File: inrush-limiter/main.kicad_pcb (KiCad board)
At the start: 2 copper layers, 24 parts, among them K1 RELAY_2RT, P1 CONN_01X06, Q1 PN2222A, Q2 PN2222A, U1 LM393

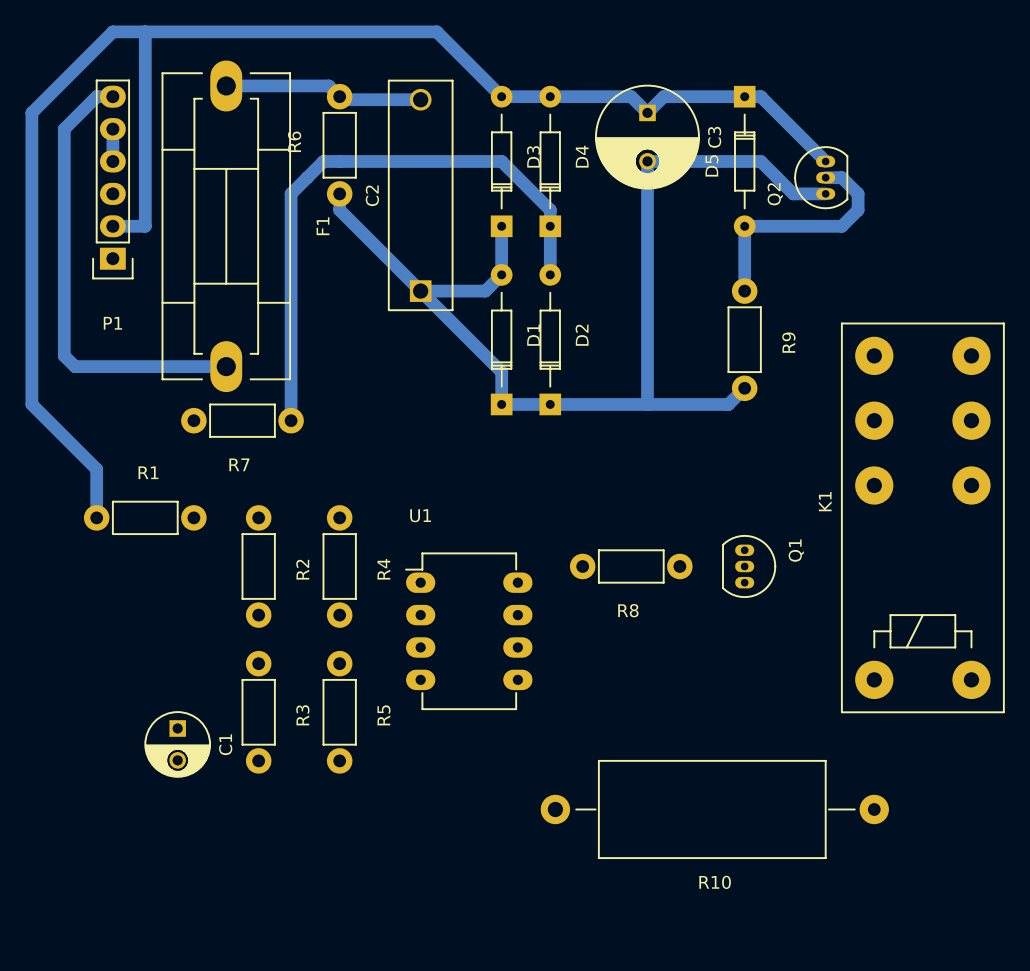
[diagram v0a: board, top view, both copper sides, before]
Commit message: update
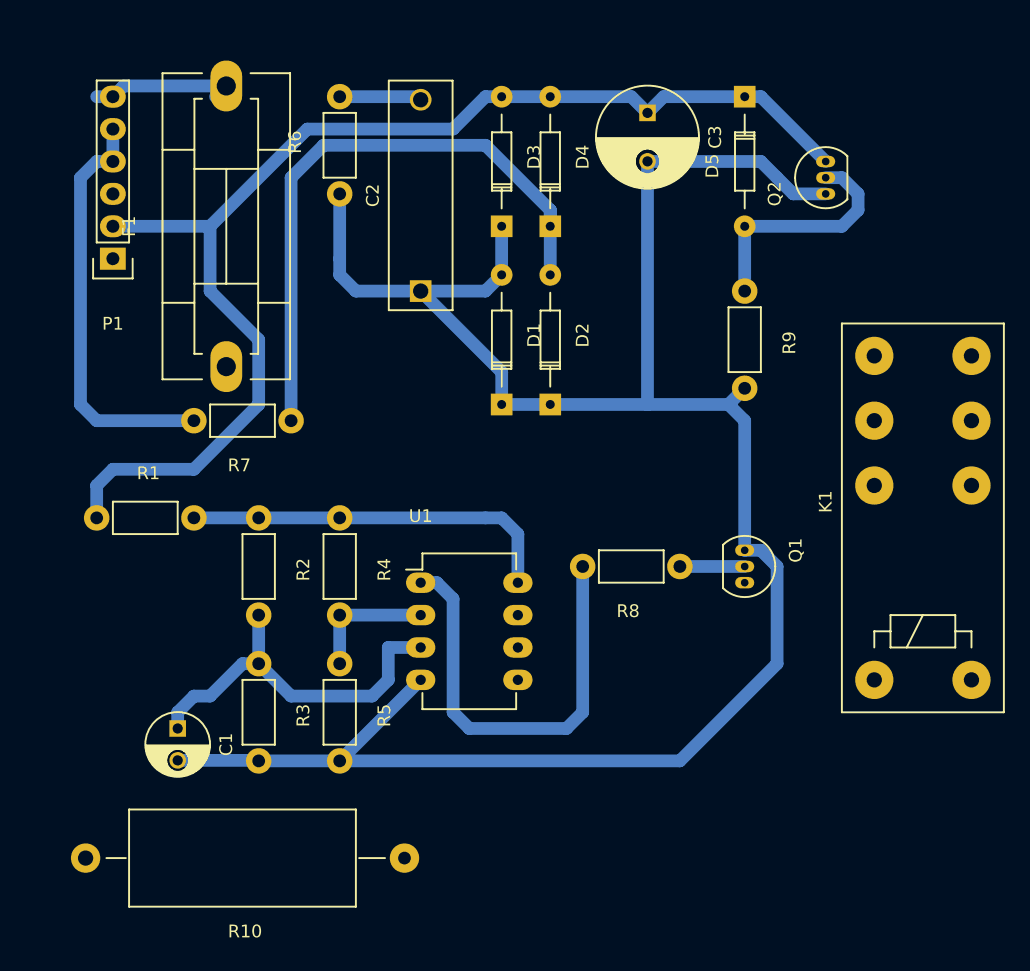
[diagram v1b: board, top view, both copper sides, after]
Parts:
- moved R10 37.0 mm to (132.1, 104.1)
- turned F1 to 90 degrees
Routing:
- net GND: track 56.2 -> 138.0 mm
- net Net-(R8-Pad2): track 0.00 -> 34.6 mm
- net AC-neut: track 2.54 -> 32.8 mm
- net Net-(C1-Pad1): track 0.00 -> 29.8 mm
- net Net-(K1-Pad9): track 0.00 -> 29.7 mm
- net +5V: track 121.8 -> 96.7 mm
- net AC-live: track 35.7 -> 11.7 mm
- net Net-(R4-Pad2): track 0.00 -> 10.2 mm
- net AC-live-f: track 15.7 -> 6.45 mm
- net Net-(Q1-Pad2): track 0.00 -> 5.08 mm
- net Net-(D2-Pad2): track 45.8 -> 48.9 mm
- net Net-(C2-Pad1): track 29.9 -> 32.9 mm
